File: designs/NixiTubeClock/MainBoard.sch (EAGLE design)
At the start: 18 parts, among them IC1 LD117ADT-TR, J1 S2B-PH-SM4, J2 S2B-PH-SM4, J3 S2B-PH-SM4, J4 S2B-PH-SM4, J5 S2B-PH-SM4, J6 S2B-PH-SM4, J7 S2B-PH-SM4

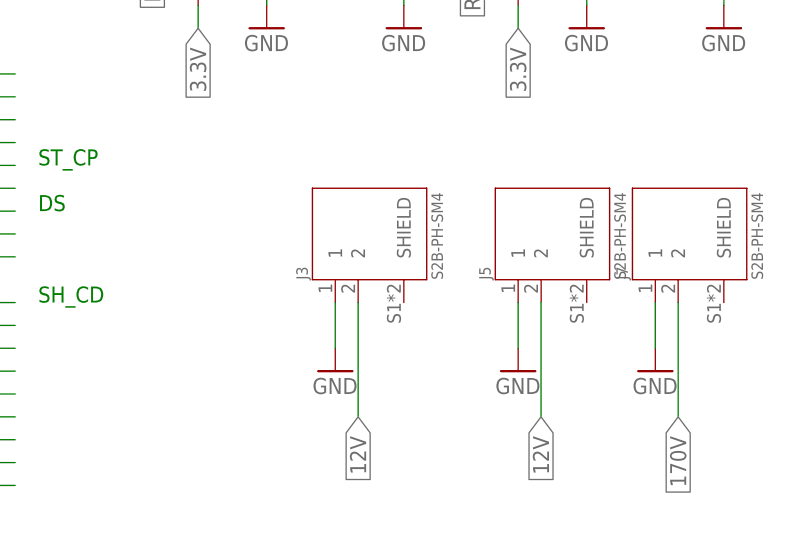
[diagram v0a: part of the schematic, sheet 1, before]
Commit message: started work on mainboard
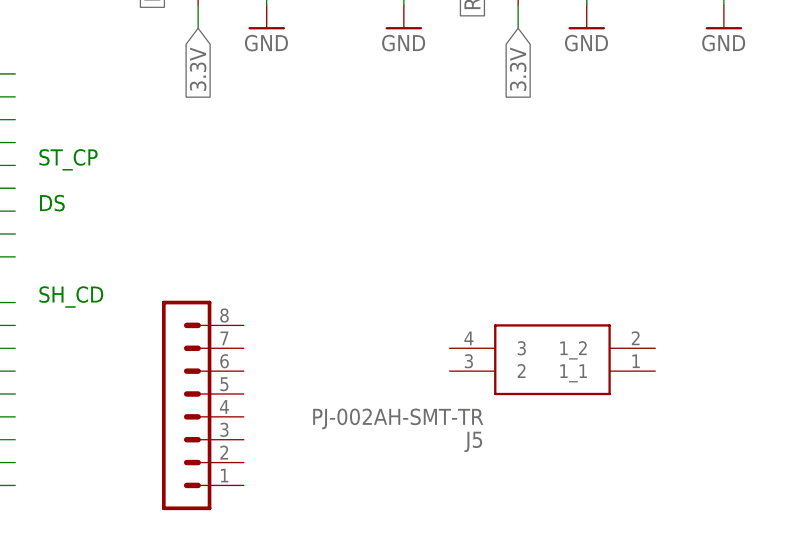
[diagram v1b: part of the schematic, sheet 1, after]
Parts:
- removed J3, J7: S2B-PH-SM4, CommonParts:S2B-PH-SM4
- added SV6: (no value), CommonParts:PINHEADER-1X8
- J5: value S2B-PH-SM4 -> PJ-002AH-SMT-TR; device CommonParts:S2B-PH-SM4 -> CommonParts:PJ-002AH-SMT-TR
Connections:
- net 12V: no longer J3.2, J5.2
- net 170V: no longer J7.2
- net GND: no longer J3.1, J5.1, J7.1
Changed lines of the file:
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@@
 <layer number="121" name="_tsilk" color="7" fill="1" visible="yes" active="yes"/>
 <layer number="122" name="_bsilk" color="7" fill="1" visible="yes" active="yes"/>
+<layer number="125" name="_tNames" color="7" fill="1" visible="no" active="yes"/>
+<layer number="127" name="Display" color="11" fill="1" visible="yes" active="yes"/>
 <layer number="131" name="prix" color="7" fill="1" visible="yes" active="yes"/>
 <layer number="132" name="test" color="7" fill="1" visible="yes" active="yes"/>
+<layer number="144" name="Drill_legend" color="7" fill="1" visible="no" active="yes"/>
 <layer number="151" name="HeatSink" color="7" fill="1" visible="yes" active="yes"/>
 <layer number="200" name="200bmp" color="7" fill="1" visible="yes" active="yes"/>
@@
 <layer number="207" name="207bmp" color="7" fill="1" visible="yes" active="yes"/>
 <layer number="208" name="208bmp" color="7" fill="1" visible="yes" active="yes"/>
+<layer number="209" name="209bmp" color="7" fill="1" visible="no" active="yes"/>
+<layer number="210" name="210bmp" color="7" fill="1" visible="no" active="yes"/>
+<layer number="211" name="211bmp" color="7" fill="1" visible="no" active="yes"/>
+<layer number="212" name="212bmp" color="7" fill="1" visible="no" active="yes"/>
+<layer number="213" name="213bmp" color="7" fill="1" visible="no" active="yes"/>
+<layer number="214" name="214bmp" color="7" fill="1" visible="no" active="yes"/>
+<layer number="215" name="215bmp" color="7" fill="1" visible="no" active="yes"/>
+<layer number="216" name="216bmp" color="7" fill="1" visible="no" active="yes"/>
+<layer number="217" name="217bmp" color="18" fill="1" visible="no" active="no"/>
+<layer number="218" name="218bmp" color="19" fill="1" visible="no" active="no"/>
+<layer number="219" name="219bmp" color="20" fill="1" visible="no" active="no"/>
+<layer number="220" name="220bmp" color="21" fill="1" visible="no" active="no"/>
+<layer number="221" name="221bmp" color="22" fill="1" visible="no" active="no"/>
+<layer number="222" name="222bmp" color="23" fill="1" visible="no" active="no"/>
+<layer number="223" name="223bmp" color="24" fill="1" visible="no" active="no"/>
+<layer number="224" name="224bmp" color="25" fill="1" visible="no" active="no"/>
 <layer number="250" name="Descript" color="7" fill="1" visible="yes" active="yes"/>
 <layer number="251" name="SMDround" color="7" fill="1" visible="yes" active="yes"/>
@@
 <part name="J4" library="CommonParts" deviceset="S2B-PH-SM4" device=""/>
 <part name="J6" library="CommonParts" deviceset="S2B-PH-SM4" device=""/>
-<part name="J5" library="CommonParts" deviceset="S2B-PH-SM4" device=""/>
-<part name="J7" library="CommonParts" deviceset="S2B-PH-SM4" device=""/>
 <part name="R1" library="CommonParts" deviceset="R-EU_1206" device="R1206" package3d_urn="urn:adsk.eagle:package:23540/2" value="10K"/>
 <part name="R2" library="CommonParts" deviceset="R-EU_1206" device="R1206" package3d_urn="urn:adsk.eagle:package:23540/2" value="10K"/>
@@
 <part name="C2" library="CommonParts" deviceset="C-EU_1206" device="C1206" package3d_urn="urn:adsk.eagle:package:23618/2"/>
 <part name="GND1" library="supply1" library_urn="urn:adsk.eagle:library:371" deviceset="GND" device=""/>
-<part name="GND7" library="supply1" library_urn="urn:adsk.eagle:library:371" deviceset="GND" device=""/>
-<part name="GND9" library="supply1" library_urn="urn:adsk.eagle:library:371" deviceset="GND" device=""/>
-<part name="J3" library="CommonParts" deviceset="S2B-PH-SM4" device=""/>
-<part name="GND5" library="supply1" library_urn="urn:adsk.eagle:library:371" deviceset="GND" device=""/>
+<part name="SV6" library="CommonParts" deviceset="PINHEADER-1X8" device="" package3d_urn="urn:adsk.eagle:package:8343/1"/>
+<part name="J5" library="CommonParts" deviceset="PJ-002AH-SMT-TR" device=""/>
 </parts>
 <sheets>
@@
 <attribute name="VALUE" x="217.70268125" y="116.83188125" size="1.275409375" layer="96" rot="R90"/>
 </instance>
-<instance part="J5" gate="G$1" x="193.04" y="71.12" smashed="yes" rot="R90">
-<attribute name="NAME" x="187.44428125" y="66.0371" size="1.272509375" layer="95" rot="R90"/>
-<attribute name="VALUE" x="202.46268125" y="66.03188125" size="1.275409375" layer="96" rot="R90"/>
-</instance>
-<instance part="J7" gate="G$1" x="208.28" y="71.12" smashed="yes" rot="R90">
-<attribute name="NAME" x="202.68428125" y="66.0371" size="1.272509375" layer="95" rot="R90"/>
-<attribute name="VALUE" x="217.70268125" y="66.03188125" size="1.275409375" layer="96" rot="R90"/>
-</instance>
 <instance part="R1" gate="G$1" x="154.94" y="101.6" smashed="yes" rot="R90">
 <attribute name="NAME" x="153.4414" y="97.79" size="1.778" layer="95" rot="R90"/>
@@
 <attribute name="VALUE" x="104.14" y="93.98" size="1.778" layer="96"/>
 </instance>
-<instance part="GND7" gate="1" x="190.5" y="55.88" smashed="yes">
-<attribute name="VALUE" x="187.96" y="53.34" size="1.778" layer="96"/>
-</instance>
-<instance part="GND9" gate="1" x="205.74" y="55.88" smashed="yes">
-<attribute name="VALUE" x="203.2" y="53.34" size="1.778" layer="96"/>
-</instance>
-<instance part="J3" gate="G$1" x="172.72" y="71.12" smashed="yes" rot="R90">
-<attribute name="NAME" x="167.12428125" y="66.0371" size="1.272509375" layer="95" rot="R90"/>
-<attribute name="VALUE" x="182.14268125" y="66.03188125" size="1.275409375" layer="96" rot="R90"/>
-</instance>
-<instance part="GND5" gate="1" x="170.18" y="55.88" smashed="yes">
-<attribute name="VALUE" x="167.64" y="53.34" size="1.778" layer="96"/>
+<instance part="SV6" gate="1" x="152.4" y="50.8" smashed="yes"/>
+<instance part="J5" gate="G$1" x="205.74" y="55.88" smashed="yes" rot="R180">
+<attribute name="NAME" x="186.69" y="48.26" size="1.778" layer="95" rot="R180" align="center-left"/>
+<attribute name="VALUE" x="186.69" y="50.8" size="1.778" layer="96" rot="R180" align="center-left"/>
 </instance>
 </instances>
@@
 <pinref part="SV1" gate="1" pin="5"/>
 </segment>
-<segment>
-<pinref part="GND7" gate="1" pin="GND"/>
-<pinref part="J5" gate="G$1" pin="1"/>
-<wire x1="190.5" y1="58.42" x2="190.5" y2="63.5" width="0.1524" layer="91"/>
-</segment>
-<segment>
-<pinref part="J7" gate="G$1" pin="1"/>
-<pinref part="GND9" gate="1" pin="GND"/>
-<wire x1="205.74" y1="58.42" x2="205.74" y2="63.5" width="0.1524" layer="91"/>
-</segment>
-<segment>
-<pinref part="GND5" gate="1" pin="GND"/>
-<pinref part="J3" gate="G$1" pin="1"/>
-<wire x1="170.18" y1="58.42" x2="170.18" y2="63.5" width="0.1524" layer="91"/>
-</segment>
 </net>
 <net name="3.3V" class="0">
@@
 </segment>
 <segment>
-<pinref part="J5" gate="G$1" pin="2"/>
-<wire x1="193.04" y1="50.8" x2="193.04" y2="63.5" width="0.1524" layer="91"/>
-<label x="193.04" y="50.8" size="1.778" layer="95" rot="R270" xref="yes"/>
-</segment>
-<segment>
 <pinref part="JP1" gate="A" pin="1"/>
 <wire x1="129.54" y1="121.92" x2="129.54" y2="116.84" width="0.1524" layer="91"/>
 <label x="129.54" y="116.84" size="1.778" layer="95" rot="R270" xref="yes"/>
 </segment>
-<segment>
-<pinref part="J3" gate="G$1" pin="2"/>
-<wire x1="172.72" y1="50.8" x2="172.72" y2="63.5" width="0.1524" layer="91"/>
-<label x="172.72" y="50.8" size="1.778" layer="95" rot="R270" xref="yes"/>
-</segment>
 </net>
 <net name="170V" class="0">
@@
 <pinref part="SV1" gate="1" pin="6"/>
 </segment>
-<segment>
-<pinref part="J7" gate="G$1" pin="2"/>
-<wire x1="208.28" y1="63.5" x2="208.28" y2="50.8" width="0.1524" layer="91"/>
-<label x="208.28" y="50.8" size="1.778" layer="95" rot="R270" xref="yes"/>
-</segment>
-</net>
+</net>
